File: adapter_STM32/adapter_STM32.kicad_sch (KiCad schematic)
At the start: 22 parts, among them J1 Conn_02x06_Top_Bottom_Mountin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, J2 Conn_02x06_Top_Bottom_Mountin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, J3 Conn_02x06_Top_Bottom_Mountin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, J4 Conn_02x06_Top_Bottom_Mountin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, U1 STM32F071CBTx, Y1 8MHz

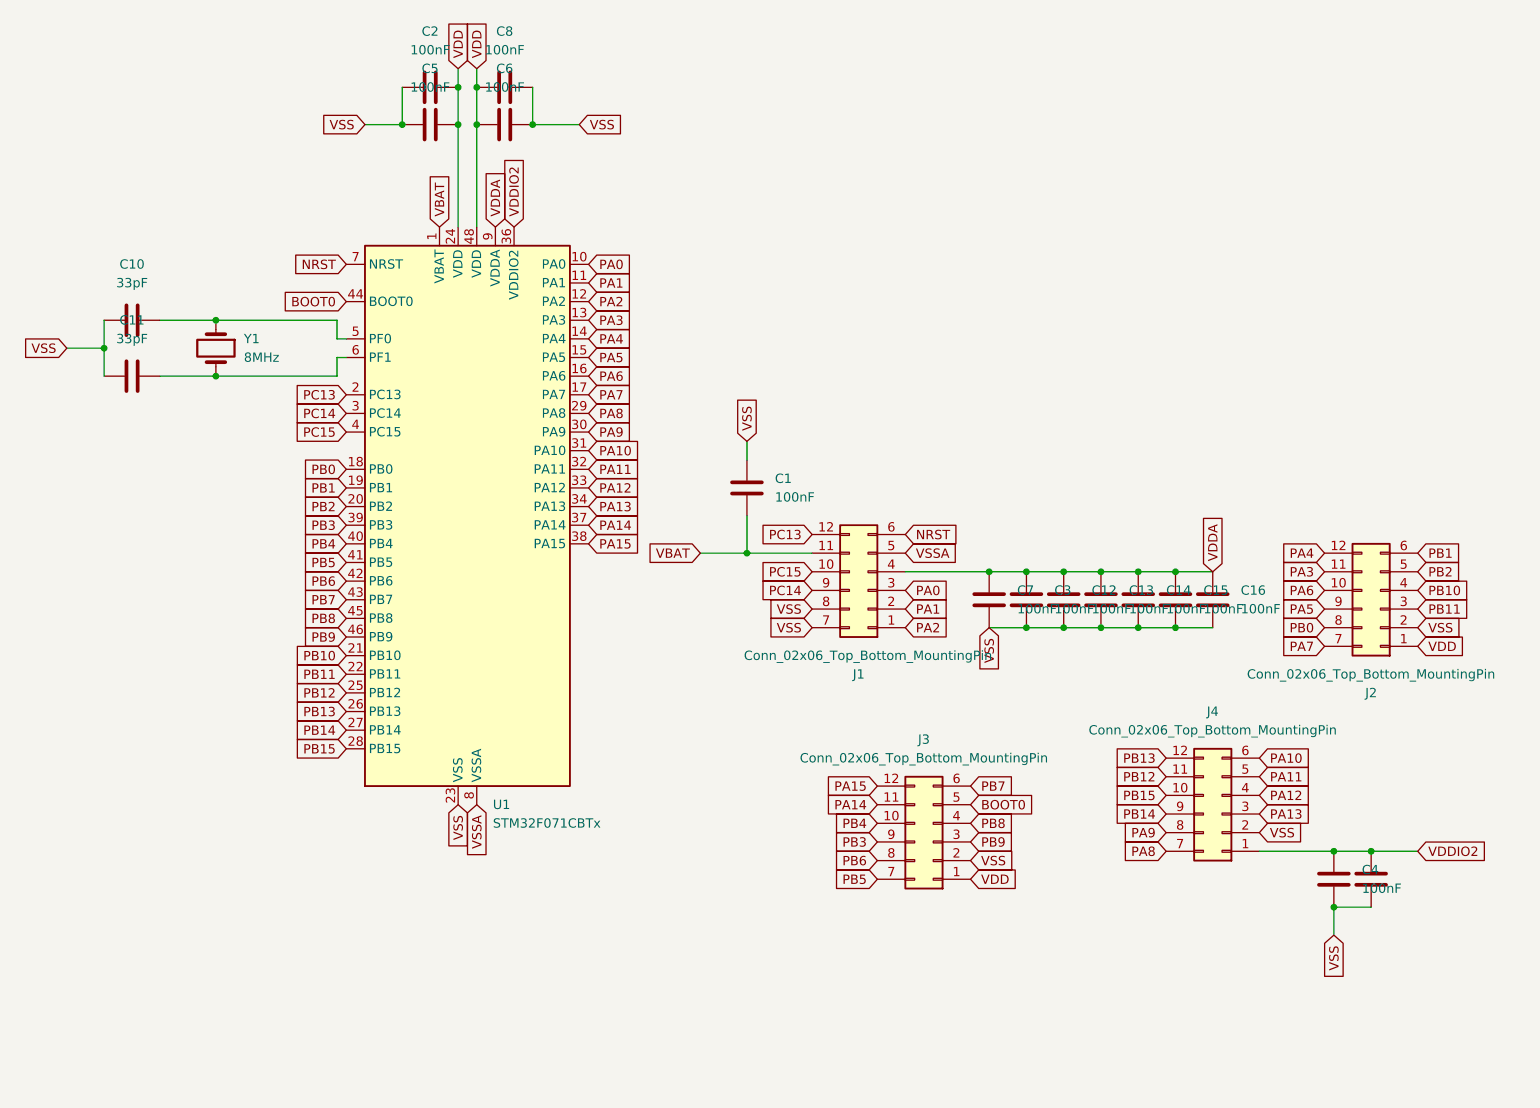
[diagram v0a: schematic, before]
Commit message: druga wersja płytki stm32 do recenzji
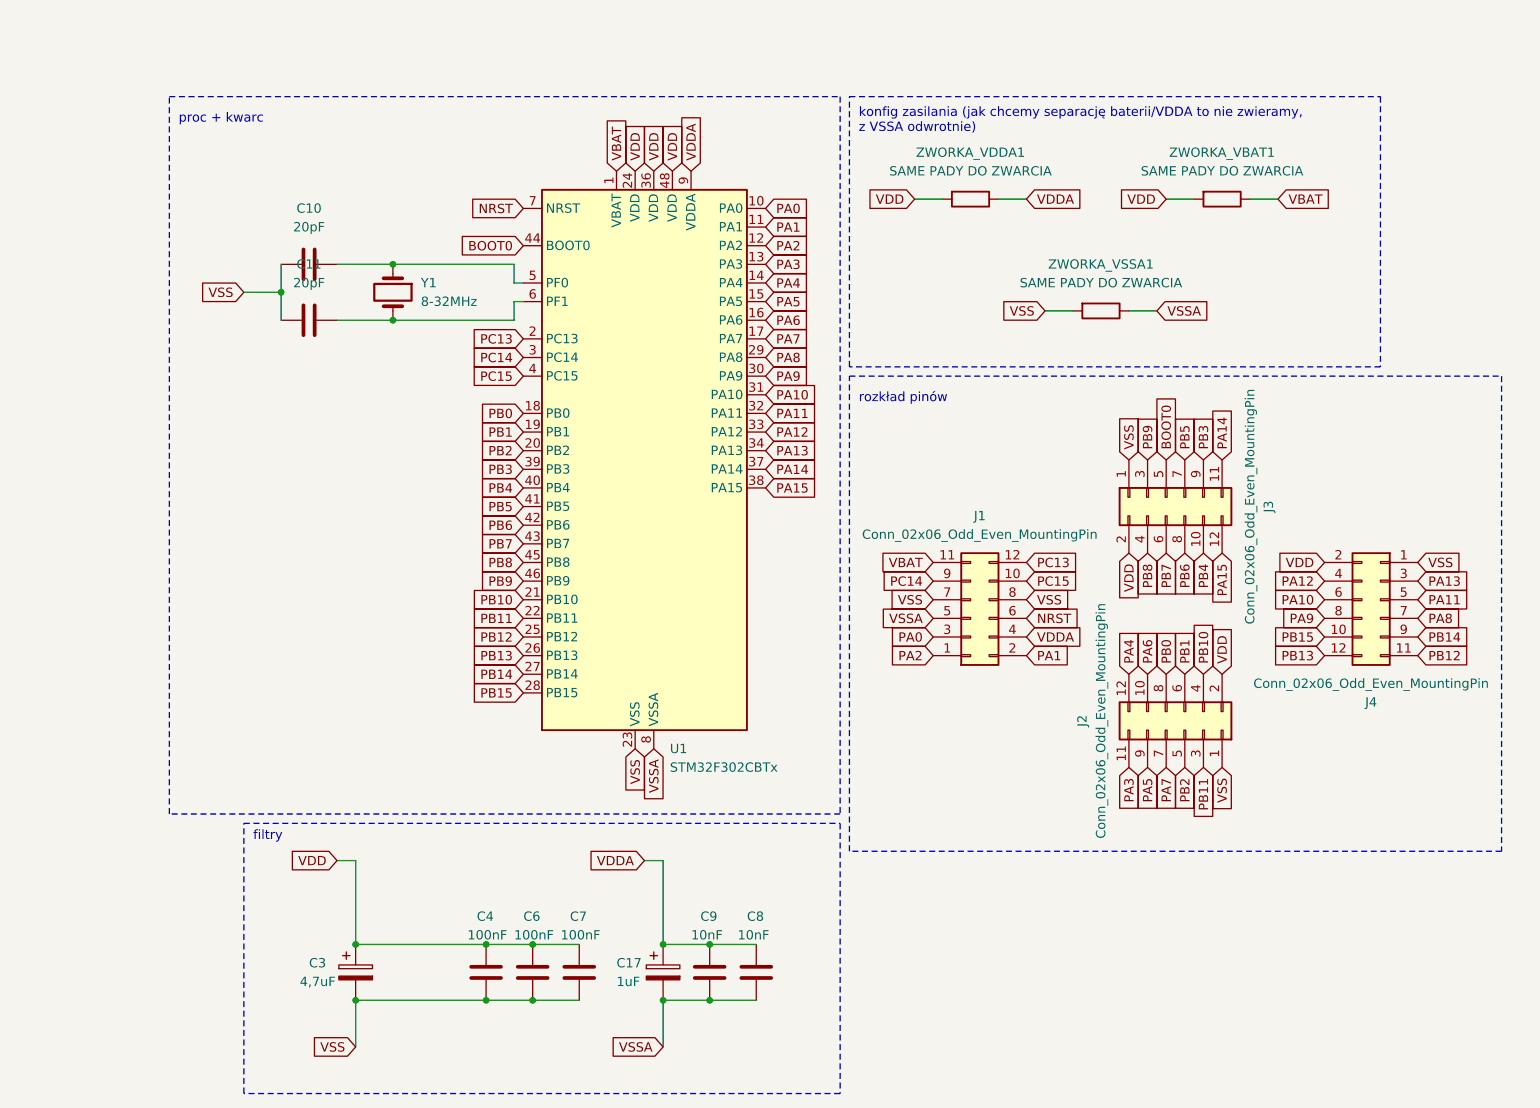
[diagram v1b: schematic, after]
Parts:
- removed C1, C12, C13, C14, C15, C16, C2, C3, C5: 100nF, Capacitor_SMD:C_0603_1608Metric, symbol Device:C
- removed J1, J2, J3, J4: Conn_02x06_Top_Bottom_MountingPin, Connector_PinHeader_2.54mm:PinHeader_2x06_P2.54mm_Vertical, symbol Connector_Generic_MountingPin:Conn_02x06_Top_Bottom_MountingPin
- removed U1: STM32F071CBTx, Package_QFP:LQFP-48_7x7mm_P0.5mm, symbol MCU_ST_STM32F0:STM32F071CBTx
- added C17: 1uF, Capacitor_THT:CP_Radial_D5.0mm_P2.00mm, symbol Device:C_Polarized
- added C3: 4,7uF, Capacitor_THT:CP_Radial_D5.0mm_P2.00mm, symbol Device:C_Polarized
- added J1, J2, J3, J4: Conn_02x06_Odd_Even_MountingPin, Connector_PinHeader_2.54mm:PinHeader_2x06_P2.54mm_Vertical, symbol Connector_Generic_MountingPin:Conn_02x06_Odd_Even_MountingPin
- added U1: STM32F302CBTx, Package_QFP:LQFP-48_7x7mm_P0.5mm, symbol MCU_ST_STM32F3:STM32F302CBTx
- added ZWORKA_VBAT1, ZWORKA_VDDA1, ZWORKA_VSSA1: SAME PADY DO ZWARCIA, Resistor_SMD:R_0201_0603Metric, symbol Device:R
- C10, C11: value 33pF -> 20pF
- C4, C6, C7: footprint Capacitor_SMD:C_0603_1608Metric -> Capacitor_SMD:C_0402_1005Metric
- C8, C9: value 100nF -> 10nF; footprint Capacitor_SMD:C_0603_1608Metric -> Capacitor_SMD:C_0402_1005Metric
- Y1: value 8MHz -> 8-32MHz
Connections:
- net BOOT0: now also J3.5 (Pin_5), U1.44 (BOOT0)
- net NRST: now also J1.6 (Pin_6), U1.7 (NRST)
- net PA0: now also J1.3 (Pin_3), U1.10 (PA0)
- net PA1: now also J1.2 (Pin_2), U1.11 (PA1)
- net PA10: now also J4.6 (Pin_6), U1.31 (PA10)
- net PA11: now also J4.5 (Pin_5), U1.32 (PA11)
- net PA12: now also J4.4 (Pin_4), U1.33 (PA12)
- net PA13: now also J4.3 (Pin_3), U1.34 (PA13)
- net PA14: now also J3.11 (Pin_11), U1.37 (PA14)
- net PA15: now also J3.12 (Pin_12), U1.38 (PA15)
- net PA2: now also J1.1 (Pin_1), U1.12 (PA2)
- net PA3: now also J2.11 (Pin_11), U1.13 (PA3)
- net PA4: now also J2.12 (Pin_12), U1.14 (PA4)
- net PA5: now also J2.9 (Pin_9), U1.15 (PA5)
- net PA6: now also J2.10 (Pin_10), U1.16 (PA6)
- net PA7: now also J2.7 (Pin_7), U1.17 (PA7)
- net PA8: now also J4.7 (Pin_7), U1.29 (PA8)
- net PA9: now also J4.8 (Pin_8), U1.30 (PA9)
- net PB0: now also J2.8 (Pin_8), U1.18 (PB0)
- net PB1: now also J2.6 (Pin_6), U1.19 (PB1)
- net PB10: now also J2.4 (Pin_4), U1.21 (PB10)
- net PB11: now also J2.3 (Pin_3), U1.22 (PB11)
- net PB12: now also J4.11 (Pin_11), U1.25 (PB12)
- net PB13: now also J4.12 (Pin_12), U1.26 (PB13)
- net PB14: now also J4.9 (Pin_9), U1.27 (PB14)
- net PB15: now also J4.10 (Pin_10), U1.28 (PB15)
- net PB2: now also J2.5 (Pin_5), U1.20 (PB2)
- net PB3: now also J3.9 (Pin_9), U1.39 (PB3)
- net PB4: now also J3.10 (Pin_10), U1.40 (PB4)
- net PB5: now also J3.7 (Pin_7), U1.41 (PB5)
- net PB6: now also J3.8 (Pin_8), U1.42 (PB6)
- net PB7: now also J3.6 (Pin_6), U1.43 (PB7)
- net PB8: now also J3.4 (Pin_4), U1.45 (PB8)
- net PB9: now also J3.3 (Pin_3), U1.46 (PB9)
- net PC13: now also J1.12 (Pin_12), U1.2 (PC13)
- net PC14: now also J1.9 (Pin_9), U1.3 (PC14)
- net PC15: now also J1.10 (Pin_10), U1.4 (PC15)
- net VBAT: now also J1.11 (Pin_11), U1.1 (VBAT), ZWORKA_VBAT1.1
- net VDD: now also C4.1, C6.1, C7.1, C3.1, J2.2 (Pin_2), J3.2 (Pin_2), J4.2 (Pin_2), U1.24 (VDD), U1.36 (VDD), U1.48 (VDD), ZWORKA_VBAT1.2, ZWORKA_VDDA1.2; no longer C6.2, C8.2
- net VDDA: now also C8.1, C9.1, C17.1, J1.4 (Pin_4), U1.9 (VDDA), ZWORKA_VDDA1.1; no longer C7.2
- net VSS: now also C4.2, C6.2, C7.2, C3.2, J1.7 (Pin_7), J1.8 (Pin_8), J2.1 (Pin_1), J3.1 (Pin_1), J4.1 (Pin_1), U1.23 (VSS), U1.35 (VSS), U1.47 (VSS), ZWORKA_VSSA1.2; no longer C4.1, C6.1, C7.1, C8.1, C9.1
- net VSSA: now also C8.2, C9.2, C17.2, J1.5 (Pin_5), U1.8 (VSSA), ZWORKA_VSSA1.1
- net at C10.1, Y1.1: now also U1.5 (PF0)
- net at C11.1, Y1.2: now also U1.6 (PF1)
- removed net VDDIO2: C4.2, C9.2
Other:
- note added: "filtry"
- note added: "konfig zasilania (jak chcemy separację baterii/VDDA to nie zwieramy, z VSSA odwrotnie)"
- note added: "proc + kwarc"
- note added: "rozkład pinów"
- moved on the sheet: C10, C11, Y1
